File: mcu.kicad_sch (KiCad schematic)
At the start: 19 parts, among them SW1 RST, SW2 BOOT, U1 ESP32-S3-WROOM-1

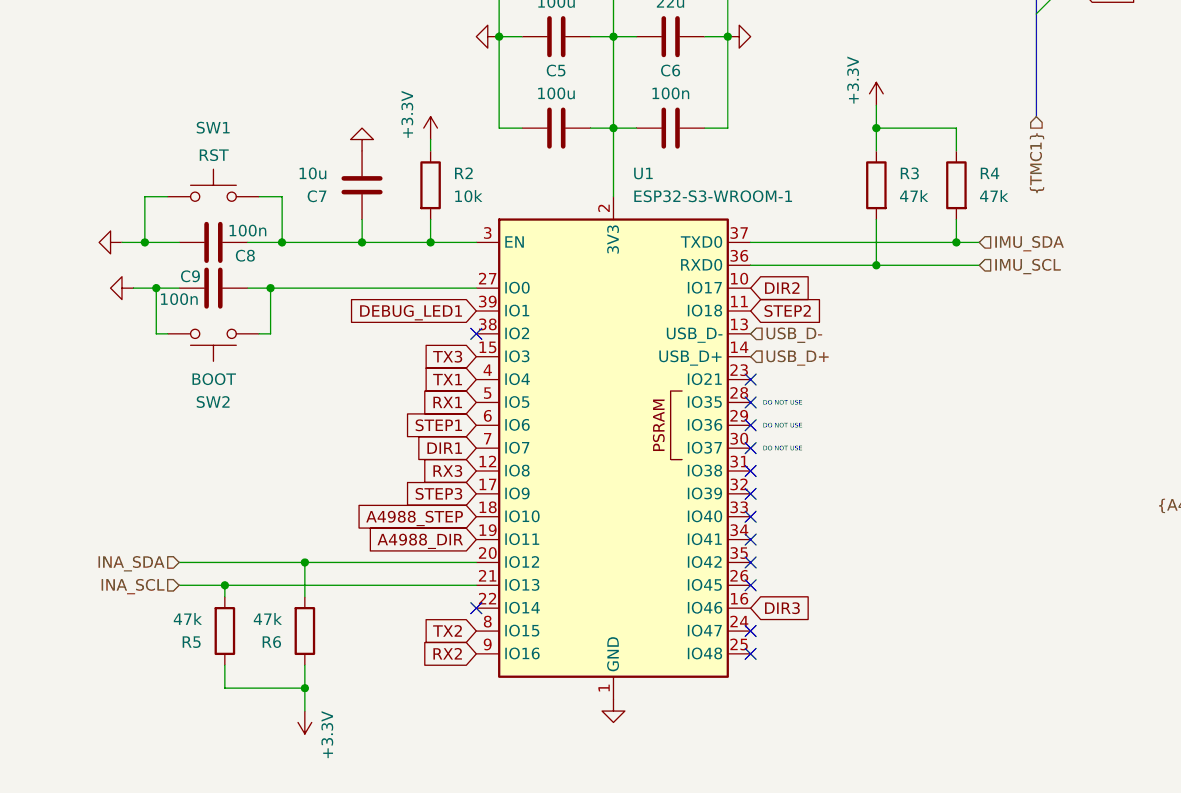
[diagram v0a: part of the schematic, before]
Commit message: Started rerouting changes
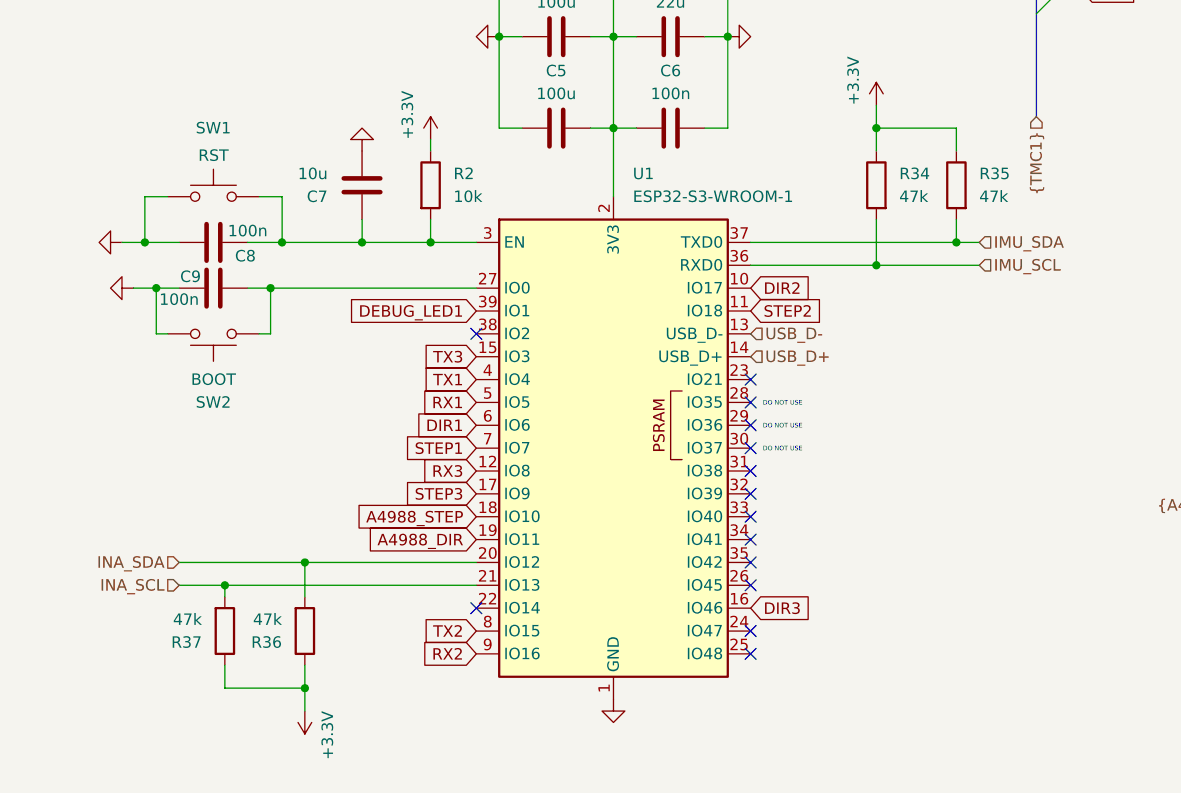
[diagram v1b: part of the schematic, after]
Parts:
- renumbered R3 to R34, R4 to R35, R6 to R36, R5 to R37
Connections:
- net DIR1: now also U1.6 (IO6); no longer U1.7 (IO7)
- net STEP1: now also U1.7 (IO7); no longer U1.6 (IO6)
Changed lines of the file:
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@@
 	(global_label "DIR1"
 		(shape input)
-		(at 105.41 110.49 180)
+		(at 105.41 107.95 180)
 		(fields_autoplaced yes)
 		(effects
@@
 		)
 		(property "Intersheetrefs" "${INTERSHEET_REFS}"
-			(at 98.0705 110.49 0)
+			(at 98.0705 107.95 0)
 			(hide yes)
 			(show_name no)
@@
 	(global_label "STEP1"
 		(shape input)
-		(at 105.41 107.95 180)
+		(at 105.41 110.49 180)
 		(fields_autoplaced yes)
 		(effects
@@
 		)
 		(property "Intersheetrefs" "${INTERSHEET_REFS}"
-			(at 96.6192 107.95 0)
+			(at 96.6192 110.49 0)
 			(hide yes)
 			(show_name no)
@@
 		(dnp no)
 		(fields_autoplaced yes)
-		(property "Reference" "R5"
+		(property "Reference" "R37"
 			(at 74.93 132.0801 0)
 			(show_name no)
@@
 			(project "Orion"
 				(path "/f9e05184-c88b-4a88-ae9c-ab2bdb32be7c/c5103ceb-5325-4a84-a025-9638a412984e/582ab2b9-8009-4dea-9a22-6d88b1b0514a"
-					(reference "R5")
+					(reference "R37")
 					(unit 1)
 				)
@@
 		(dnp no)
 		(fields_autoplaced yes)
-		(property "Reference" "R3"
+		(property "Reference" "R34"
 			(at 152.4 80.0099 0)
 			(show_name no)
@@
 			(project "Orion"
 				(path "/f9e05184-c88b-4a88-ae9c-ab2bdb32be7c/c5103ceb-5325-4a84-a025-9638a412984e/582ab2b9-8009-4dea-9a22-6d88b1b0514a"
-					(reference "R3")
+					(reference "R34")
 					(unit 1)
 				)
@@
 		(dnp no)
 		(fields_autoplaced yes)
-		(property "Reference" "R4"
+		(property "Reference" "R35"
 			(at 161.29 80.0099 0)
 			(show_name no)
@@
 			(project "Orion"
 				(path "/f9e05184-c88b-4a88-ae9c-ab2bdb32be7c/c5103ceb-5325-4a84-a025-9638a412984e/582ab2b9-8009-4dea-9a22-6d88b1b0514a"
-					(reference "R4")
+					(reference "R35")
 					(unit 1)
 				)
@@
 		(dnp no)
 		(fields_autoplaced yes)
-		(property "Reference" "R6"
+		(property "Reference" "R36"
 			(at 83.82 132.0801 0)
 			(show_name no)
@@
 			(project "Orion"
 				(path "/f9e05184-c88b-4a88-ae9c-ab2bdb32be7c/c5103ceb-5325-4a84-a025-9638a412984e/582ab2b9-8009-4dea-9a22-6d88b1b0514a"
-					(reference "R6")
+					(reference "R36")
 					(unit 1)
 				)
